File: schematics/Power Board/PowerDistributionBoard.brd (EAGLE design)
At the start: 66 x 53.3 mm, 11 parts

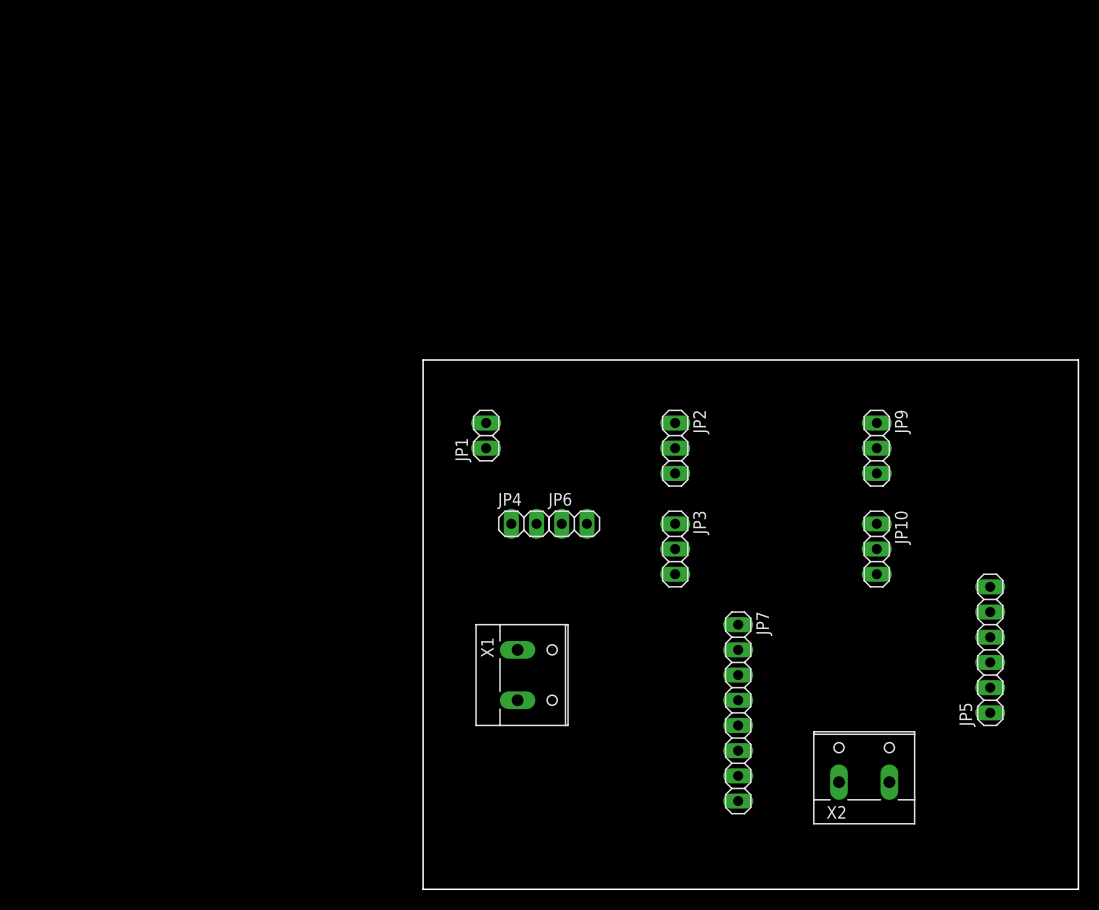
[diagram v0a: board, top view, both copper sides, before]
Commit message: Final Board Sent for Fabrication
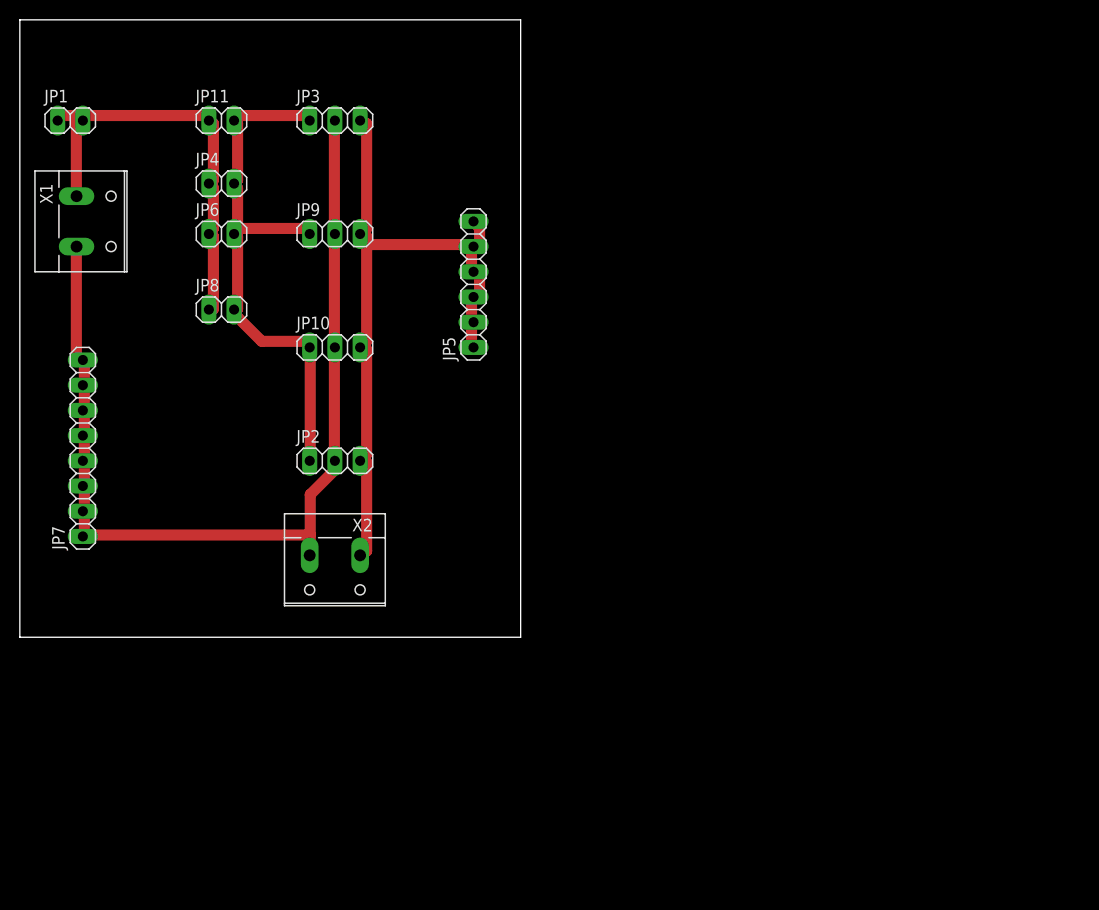
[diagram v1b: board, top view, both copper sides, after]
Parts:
- added JP11, JP8: (no value), pinhead:1X02
- moved JP7 71.2 mm to (6.35, 35.6), turned to 90 degrees
- moved JP5 63.8 mm to (45.7, 52.1)
- moved X1 63.8 mm to (6.35, 58.4)
- moved JP9 58.7 mm to (31.8, 57.1), turned to 0 degrees
- moved JP10 58.3 mm to (31.8, 45.7), turned to 0 degrees
- moved X2 57.5 mm to (31.8, 24.1), turned to 180 degrees
- moved JP3 55.1 mm to (31.8, 68.6), turned to 0 degrees
- moved JP1 52.6 mm to (5.08, 68.6), turned to 0 degrees
- moved JP6 46.0 mm to (20.3, 57.1)
- moved JP4 45.9 mm to (20.3, 62.2)
- moved JP2 34.3 mm to (31.8, 34.3), turned to 0 degrees
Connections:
- removed net N$2: JP4.2, JP6.1
- removed net V-IN: JP10.1, JP2.1, JP3.1, JP6.2, JP9.1
- new net V-IN1: JP10.1, JP11.2, JP2.1, JP3.1, JP4.2, JP6.2, JP8.2, JP9.1
- net N$1: now also JP11.1, JP6.1, JP8.1
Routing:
- net COMMON-GND: track 0.00 -> 97.9 mm
- net SENSOR-5V+: track 0.00 -> 73.3 mm
- net V-IN1: track 0.00 -> 57.6 mm
- net N$1: track 0.00 -> 45.0 mm
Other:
- board size 66 x 53.3 mm -> 50.5 x 62.2 mm
